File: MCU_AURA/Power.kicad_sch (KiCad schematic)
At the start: 65 parts, among them J100 XT30PW-M, J101 USB_C_Receptacle_USB2.0_16P, U100 TPS56C230RJER, U101 SI4825DDY-T1-GE3, U102 TPS2115ADRBR, U103 TLV62566DBVR, U104 AP2127N-1.8

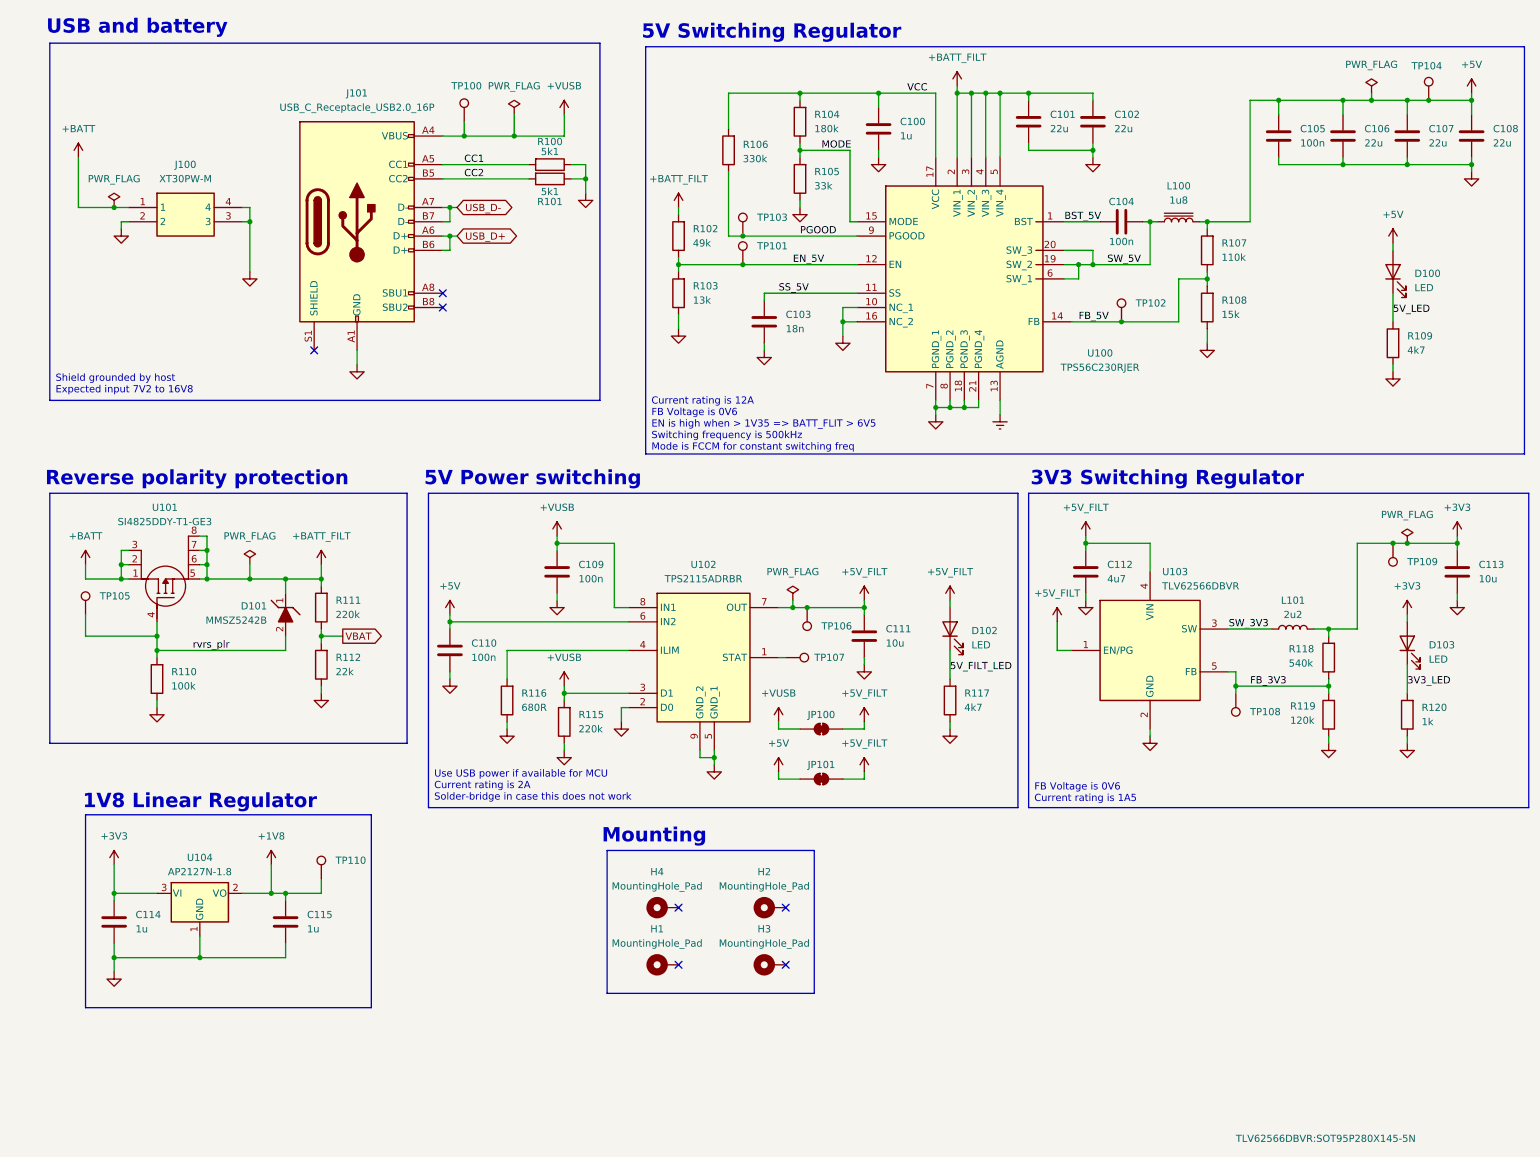
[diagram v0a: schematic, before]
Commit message: Synchronised
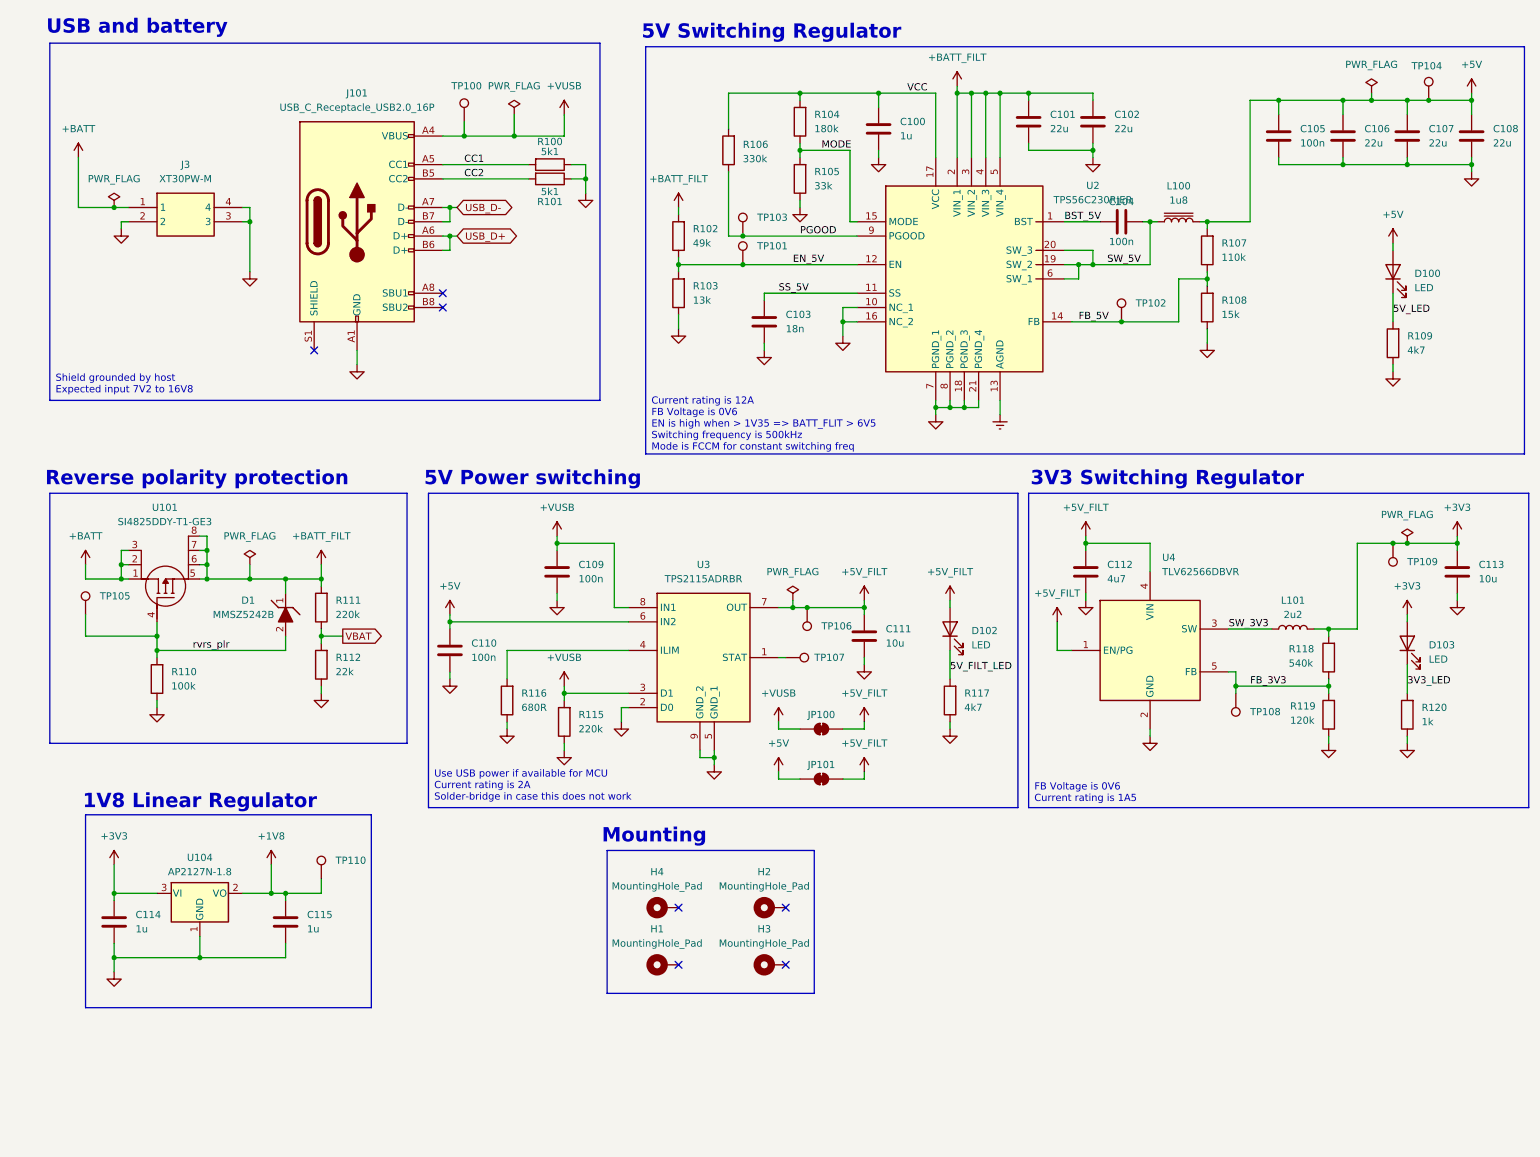
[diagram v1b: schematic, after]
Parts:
- removed D101: MMSZ5242B, MMSZ5252B:MMSZ5252B, symbol SamacSys_Parts:MMSZ5242B
- removed J100: XT30PW-M, XT30PWM, symbol XT30PW-M:XT30PW-M
- removed U100: TPS56C230RJER, TPS56C230RJER:QFN45P300X300X100-21N-D, symbol SamacSys_Parts:TPS56C230RJER
- removed U102: TPS2115ADRBR, TPS2115ADRBR:SON65P300X300X100-9N-D, symbol SamacSys_Parts:TPS2115ADRBR
- removed U103: TLV62566DBVR, TLV62566DBVR:SOT95P280X145-5N, symbol SamacSys_Parts:TLV62566DBVR
- added D1: MMSZ5242B, MMSZ5252B:MMSZ5252B, symbol MMSZ5252B:MMSZ5242B
- added J3: XT30PW-M, XT30PWM:XT30PWM, symbol XT30PW-M:XT30PW-M
- added U2: TPS56C230RJER, TPS56C230RJER:QFN45P300X300X100-21N-D, symbol TPS56C230RJER:TPS56C230RJER
- added U3: TPS2115ADRBR, TPS2115ADRBR:SON65P300X300X100-9N-D, symbol TPS2115ADRBR:TPS2115ADRBR
- added U4: TLV62566DBVR, TLV62566DBVR:SOT95P280X145-5N, symbol TLV62566DBVR:TLV62566DBVR
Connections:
- net +5V: now also U3.6 (IN2)
- net +5V_FILT: now also U3.7 (OUT), U4.1 (EN/PG), U4.4 (VIN)
- net +BATT: now also J3.1
- net +BATT_FILT: now also D1.1 (K), U2.2 (VIN_1), U2.3 (VIN_2), U2.4 (VIN_3), U2.5 (VIN_4)
- net +VUSB: now also U3.3 (D1), U3.8 (IN1)
- net BST_5V: now also U2.1 (BST)
- net EN_5V: now also U2.12 (EN)
- net FB_3V3: now also U4.5 (FB)
- net FB_5V: now also U2.14 (FB)
- net GND: now also J3.2, J3.3, J3.4, U2.10 (NC_1), U2.16 (NC_2), U2.18 (PGND_3), U2.21 (PGND_4), U2.7 (PGND_1), U2.8 (PGND_2), U3.2 (D0), U3.5 (GND_1), U3.9 (GND_2), U4.2 (GND)
- net GNDREF: now also U2.13 (AGND)
- net MODE: now also U2.15 (MODE)
- net PGOOD: now also U2.9 (PGOOD)
- net SS_5V: now also U2.11 (SS)
- net SW_3V3: now also U4.3 (SW)
- net SW_5V: now also U2.19 (SW_2), U2.20 (SW_3), U2.6 (SW_1)
- net VCC: now also U2.17 (VCC)
- net rvrs_plr: now also D1.2 (A)
- net at R116.2: now also U3.4 (ILIM)
- net at TP107.1: now also U3.1 (STAT)
